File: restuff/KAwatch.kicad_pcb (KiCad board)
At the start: 2 copper layers, 56 x 78 mm, 24 parts, among them J1 Conn_01x08, J2 USB_C_Receptacle_PowerOnly_6P, J3 Conn_01x02, J4 Conn_01x02, Q1 Q_NPN_BCE, SW1 SW_Push, U1 ESP32-WROOM-32E, U2 MCP73831-2-OT, U3 XC6220B331MR

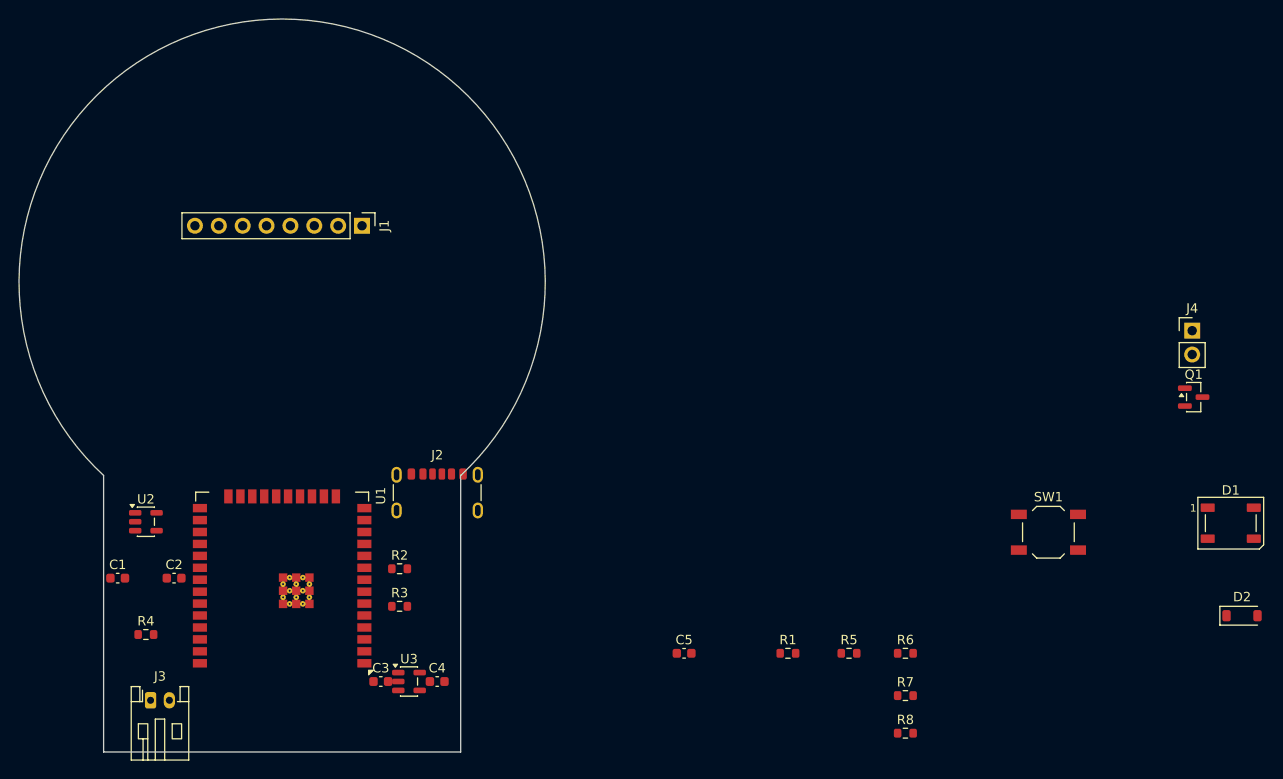
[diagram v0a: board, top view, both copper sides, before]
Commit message: compacting pcb
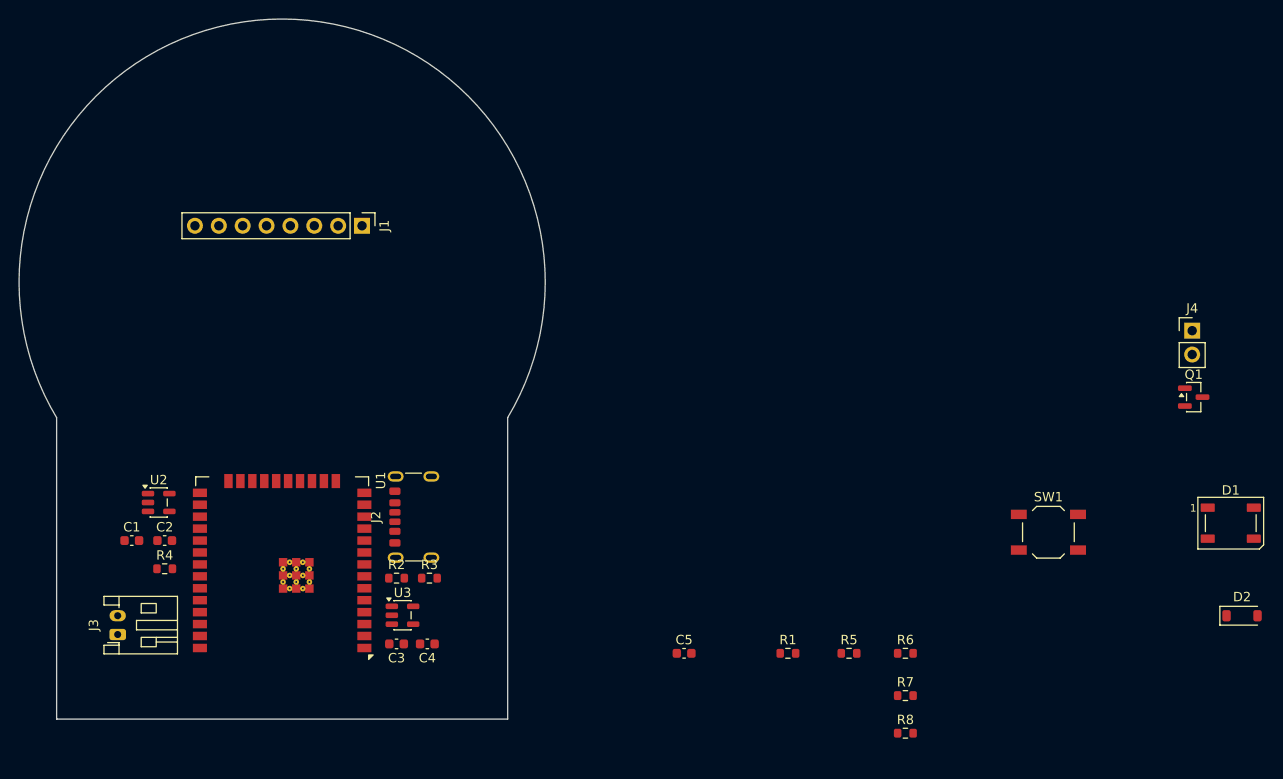
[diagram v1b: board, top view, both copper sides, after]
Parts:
- moved J3 7.83 mm to (101.0, 132.0), turned to 90 degrees
- moved R4 7.28 mm to (106.0, 125.0)
- moved U3 7.08 mm to (131.3, 129.9)
- moved R3 4.37 mm to (134.2, 126.0)
- moved C3 4.34 mm to (130.7, 133.0)
- moved C1 4.27 mm to (102.5, 122.0)
- moved C4 4.14 mm to (133.9, 133.0)
- moved C2 4.12 mm to (106.0, 122.0)
- moved U2 2.46 mm to (105.4, 118.0)
- moved J2 2.07 mm to (133.6, 119.5), turned to 90 degrees
- moved U1 1.63 mm to (118.5, 128.2)
- moved R2 1.05 mm to (130.7, 126.0)
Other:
- board size 56 x 78 mm -> 56 x 74.5 mm

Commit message: pcb edits and routing start
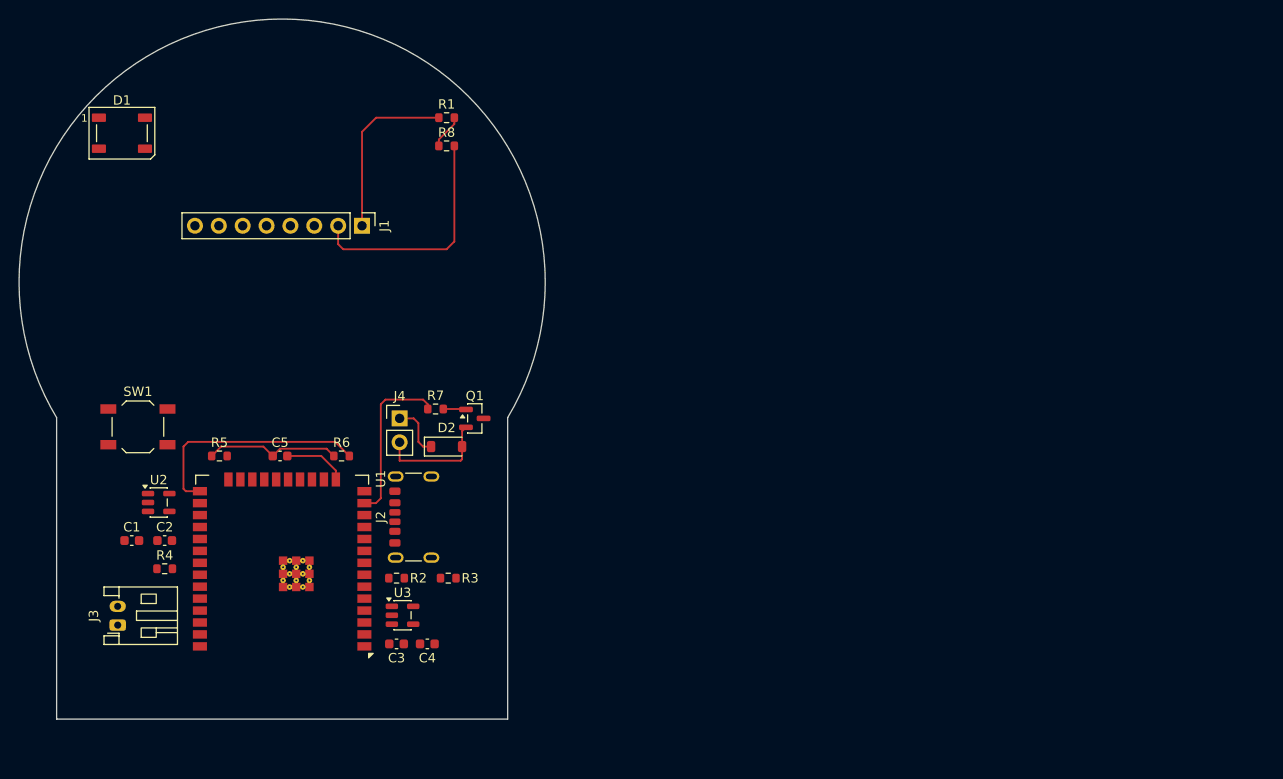
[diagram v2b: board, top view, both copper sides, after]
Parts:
- moved D1 125.1 mm to (101.5, 78.7)
- moved SW1 97.5 mm to (103.2, 109.9)
- moved D2 86.5 mm to (136.0, 112.0)
- moved J4 84.9 mm to (131.0, 109.0)
- moved R8 79.3 mm to (136.0, 80.0)
- moved Q1 76.5 mm to (139.0, 109.0)
- moved R5 70.2 mm to (111.8, 113.0)
- moved R1 67.6 mm to (136.0, 77.0)
- moved R6 63.6 mm to (124.8, 113.0)
- moved R7 58.6 mm to (134.8, 108.0)
- moved C5 47.9 mm to (118.3, 113.0)
- moved R3 2.00 mm to (136.2, 126.0)
- moved J3 1.00 mm to (101.0, 131.0)
- moved U1 0.17 mm to (118.5, 128.0)
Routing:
- net /+3V3: track 0.00 -> 39.0 mm
- net GND: track 0.00 -> 32.0 mm
- net Net-(U1-IO0): track 0.00 -> 24.8 mm
- net Net-(U1-IO14): track 0.00 -> 17.9 mm
- net Net-(D2-A): track 0.00 -> 12.2 mm
- net Net-(U1-IO34): track 0.00 -> 3.68 mm
- net Net-(Q1-B): track 0.00 -> 2.43 mm
